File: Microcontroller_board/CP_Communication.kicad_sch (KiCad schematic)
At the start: 13 parts, among them J5 CAR_CONNECTOR, U5 LM324

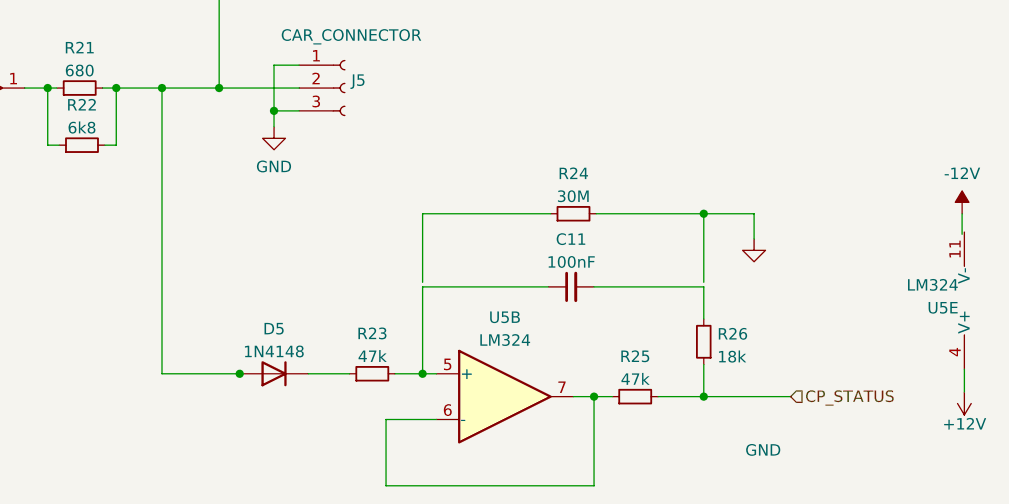
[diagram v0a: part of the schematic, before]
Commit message: Upload
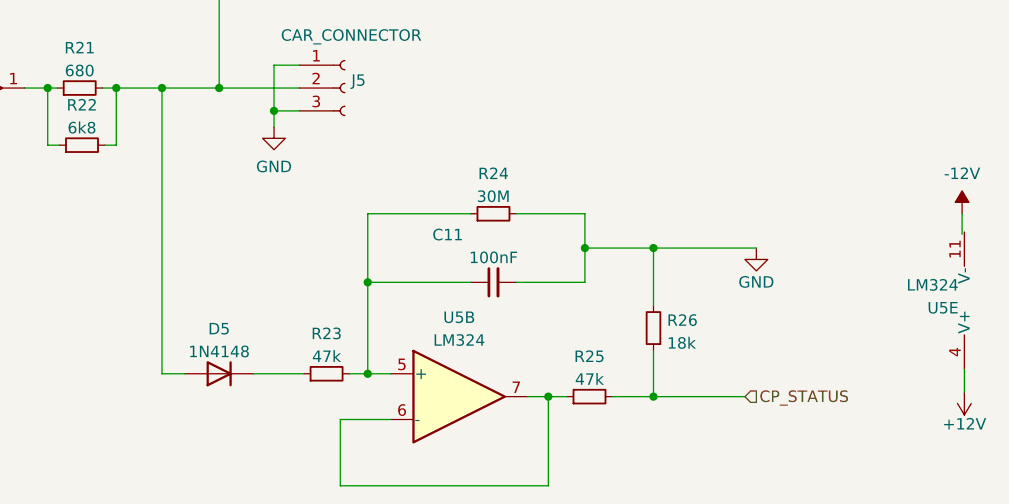
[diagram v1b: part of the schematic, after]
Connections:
- net GND: now also C11.2, R26.2
- net at R24.1: now also C11.1, R23.2, U5.5 (+)
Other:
- moved on the sheet: C11, D5, R23, R24, R25, R26, U5B
